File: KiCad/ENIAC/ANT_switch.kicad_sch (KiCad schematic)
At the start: 13 parts, among them J4 Conn_Coaxial, U8 4259-63

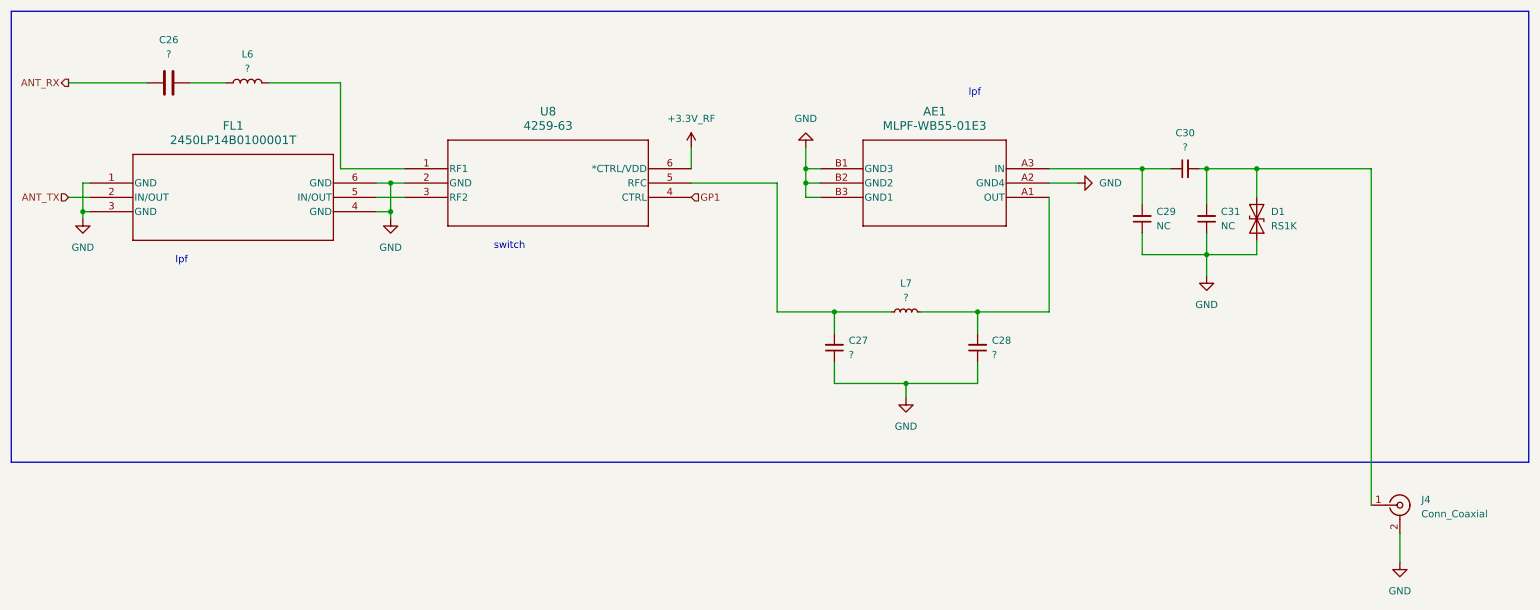
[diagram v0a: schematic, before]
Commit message: john d tickle
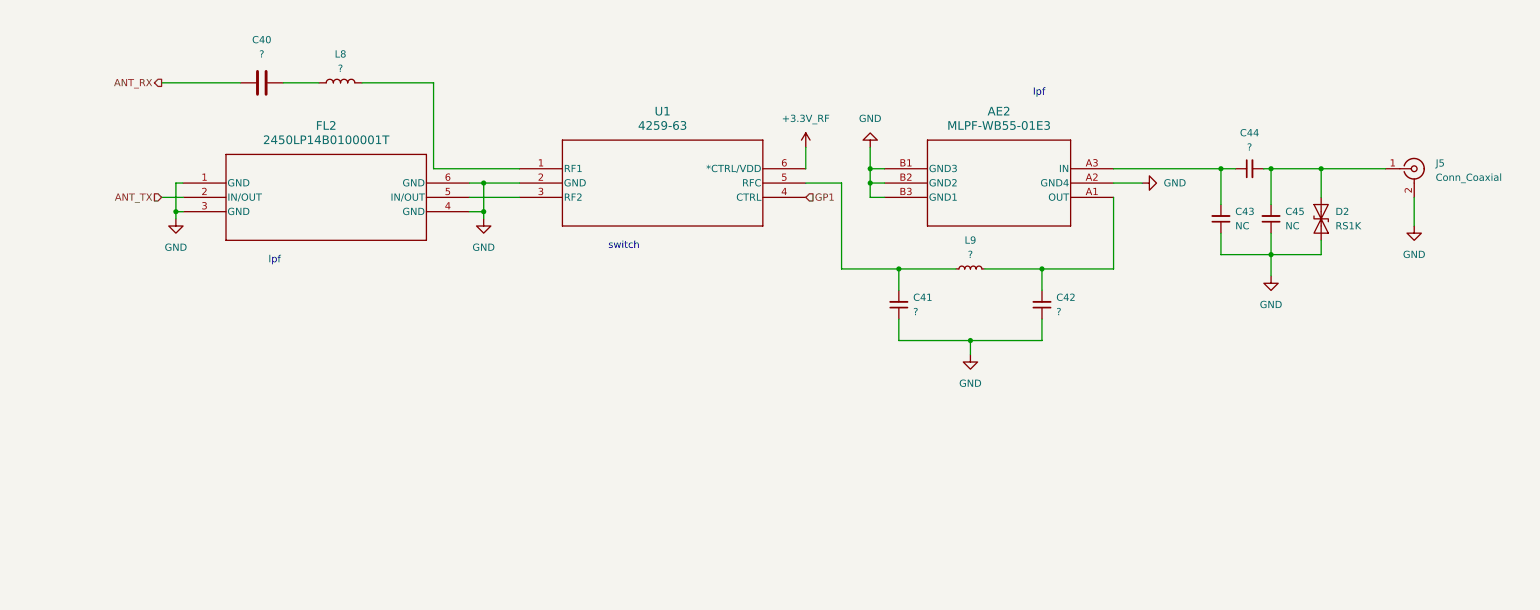
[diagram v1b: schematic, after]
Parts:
- renumbered AE1 to AE2, C26 to C40, C27 to C41, C28 to C42, C29 to C43, C30 to C44, C31 to C45, D1 to D2, FL1 to FL2, J4 to J5, L6 to L8, L7 to L9, U8 to U1
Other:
- moved on the sheet: AE2, C40, C41, C42, C43, C44, C45, D2, FL2, J5, L8, L9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

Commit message: funny commit message
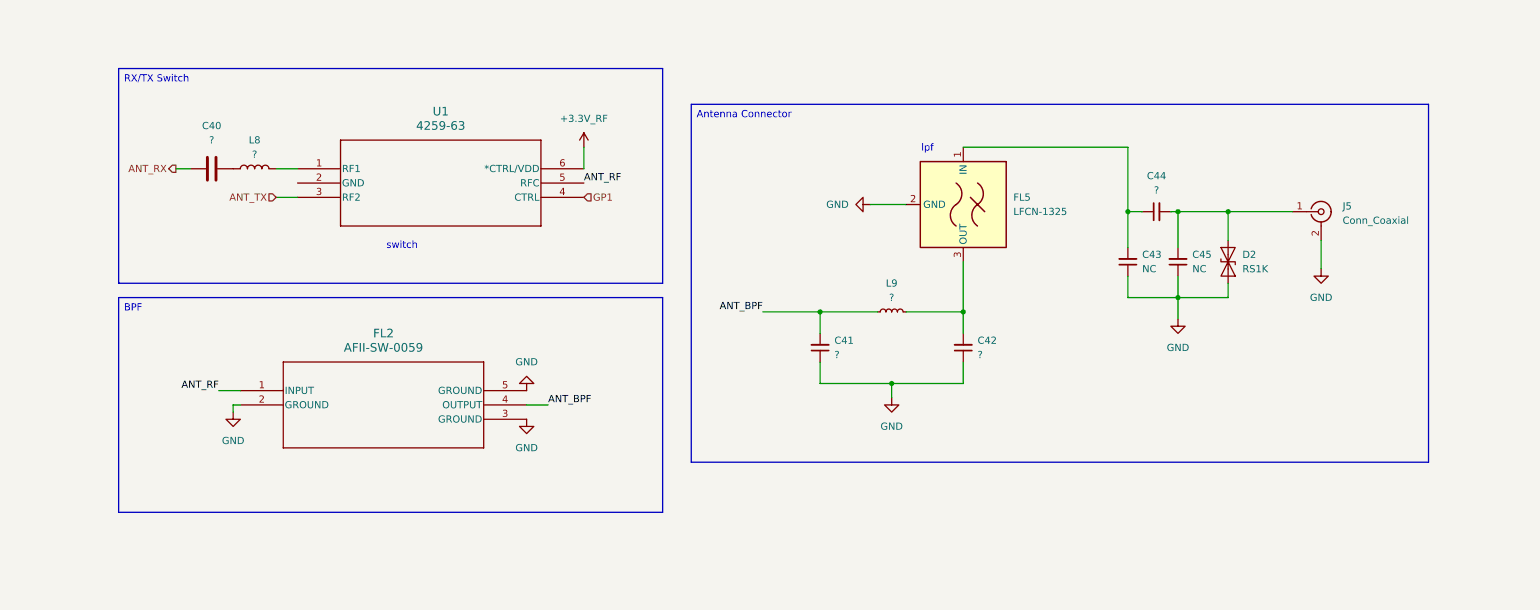
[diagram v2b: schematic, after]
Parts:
- removed AE2: MLPF-WB55-01E3, MLPF-WB55-01E3_STM, symbol 2025-11-10_00-22-04:MLPF-WB55-01E3
- removed FL2: 2450LP14B0100001T, 3550LP_JOT, symbol 2025-11-10_17-30-01:3550LP14A0300001T
- added FL2: AFII-SW-0059, SMD5_SAW-B7520_QUA, symbol 2026-03-09_02-05-18:B39242B7520P810
- added FL5: LFCN-1325, Filter:Filter_Mini-Circuits_FV1206, symbol RF_Filter:LFCN-1325
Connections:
- net ANT_TX: now also U1.3 (RF2)
- net GND: now also FL2.2 (GROUND), FL2.3 (GROUND), FL2.5 (GROUND), FL5.2 (GND), FL5.4 (GND); no longer U1.2 (GND)
- net ANT_BPF: now reaches C41.2, L9.1
- net ANT_BPF: now also FL2.4 (OUTPUT); no longer U1.5 (RFC)
- net at C42.2, L9.2: now also FL5.3 (OUT)
- net at C43.2, C44.1: now also FL5.1 (IN)
- new net ANT_RF: FL2.1 (INPUT), U1.5 (RFC)
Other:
- moved on the sheet: C40, C41, C42, C43, C44, C45, D2, J5, L8, L9, U1
